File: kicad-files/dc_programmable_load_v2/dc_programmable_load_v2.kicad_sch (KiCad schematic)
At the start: 43 parts, among them J1 DC Jack 12V, J3 Conn_01x04_Socket, Q1 IRF3205, U1 LM358DR, U2 ER_OLEDM0.91_1x-I2C, U3 AP63200WU, U4 DS18B20, U5 S-2050

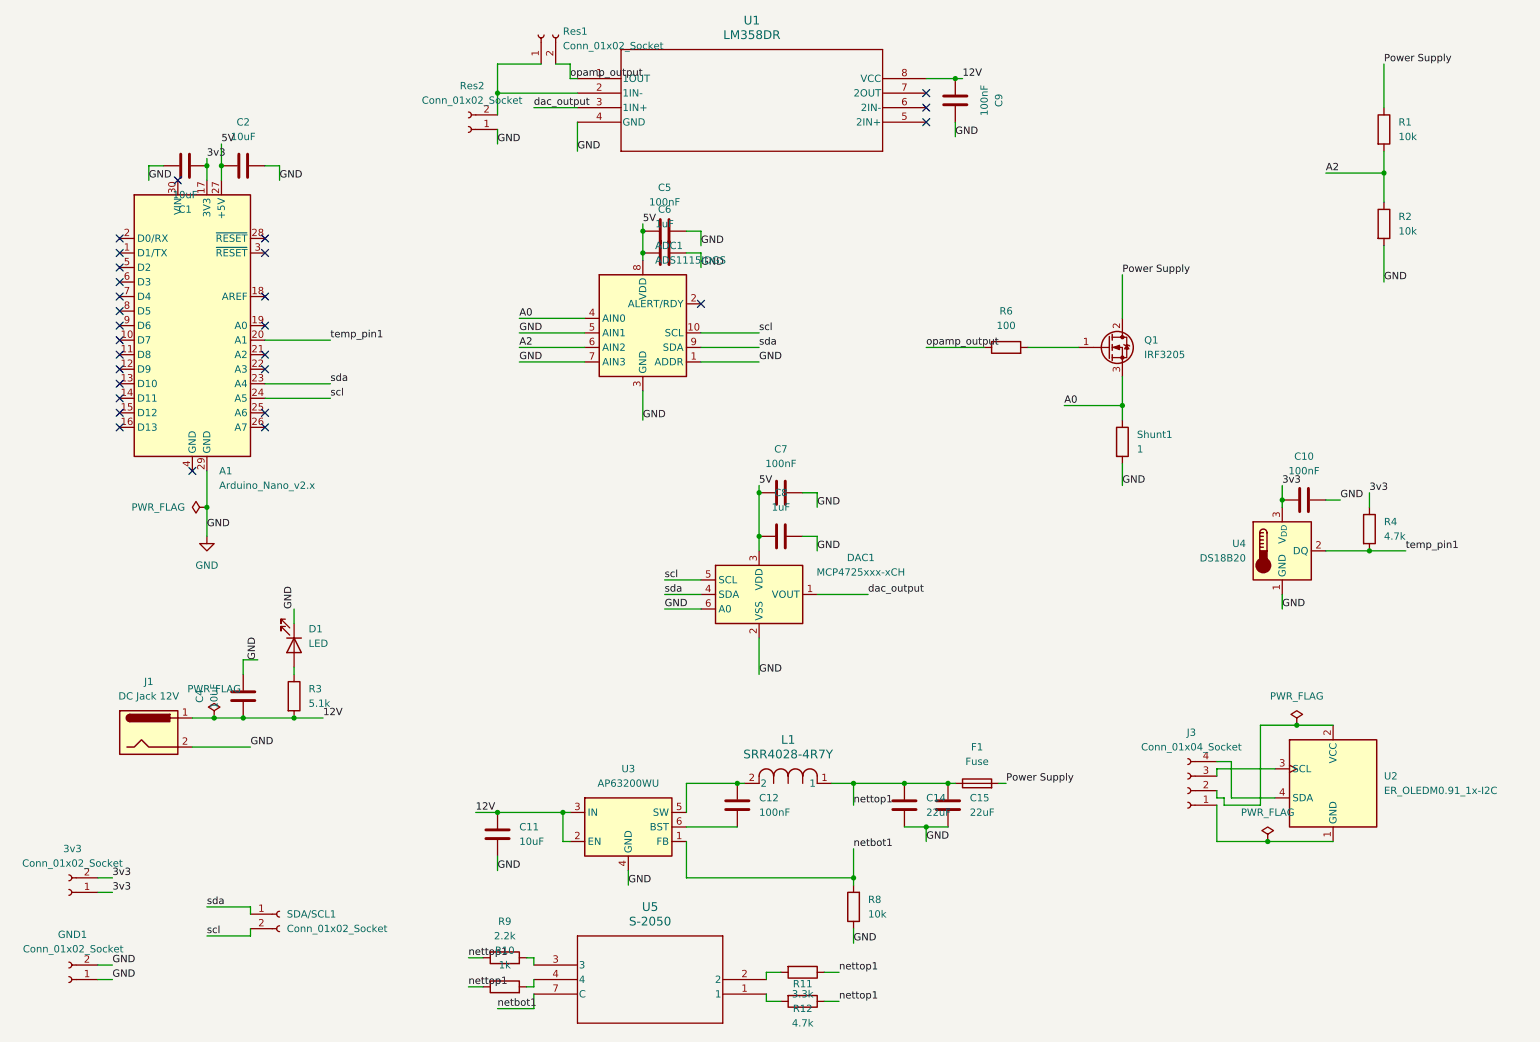
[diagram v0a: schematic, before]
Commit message: anand newest edits
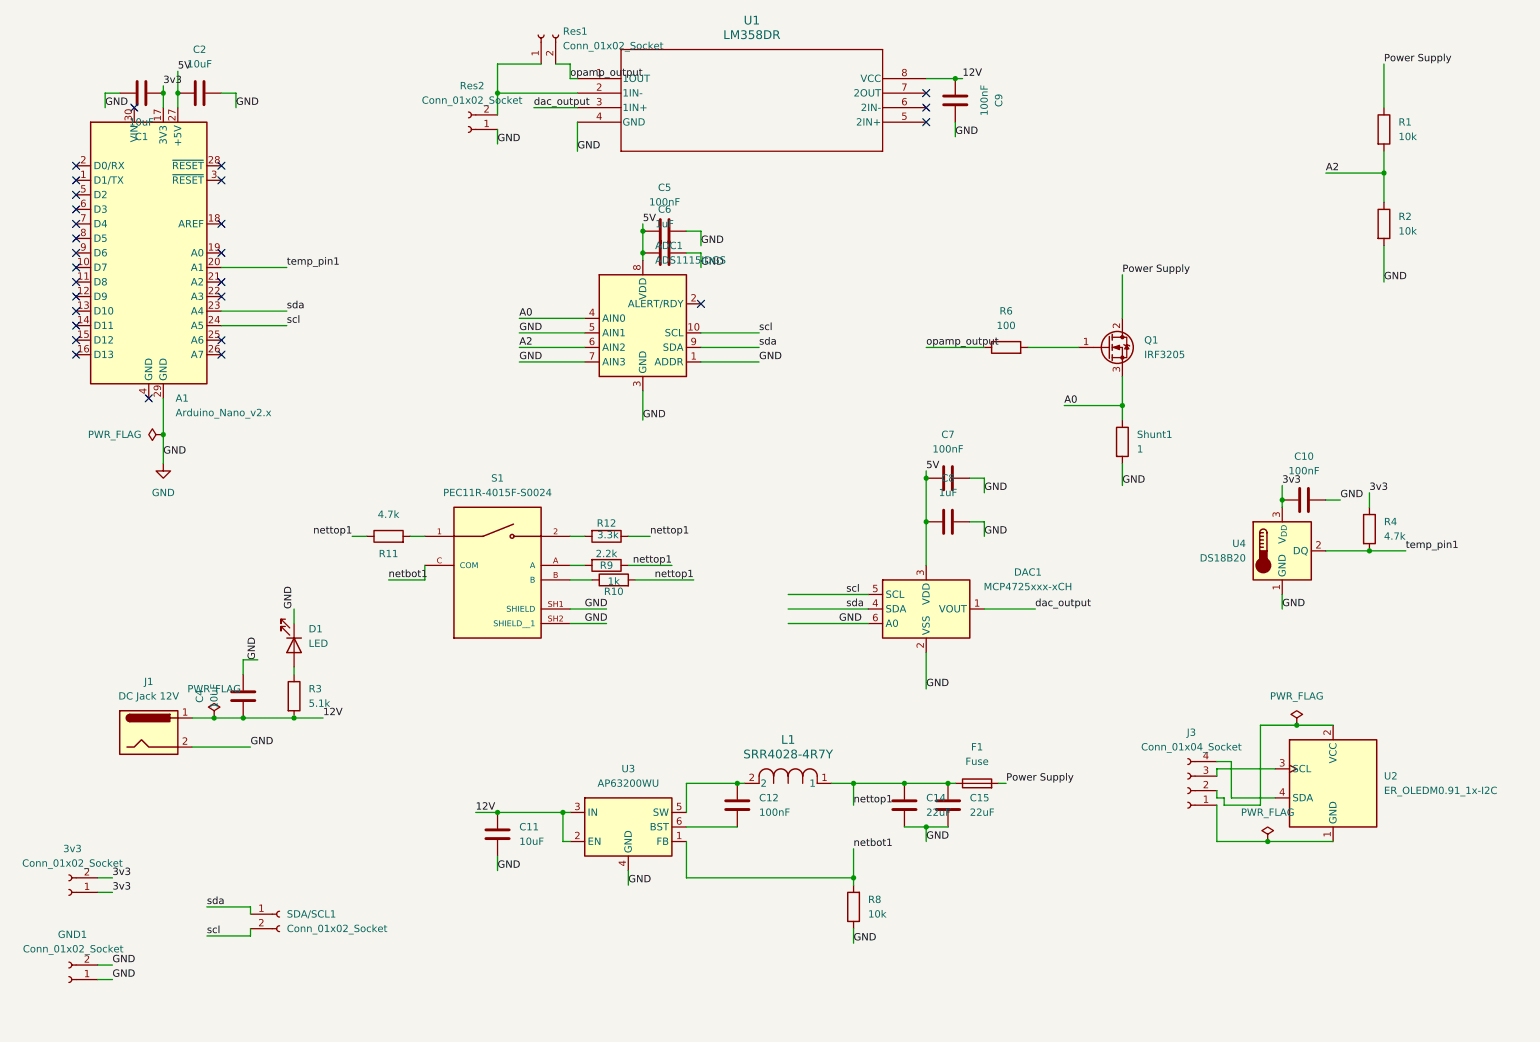
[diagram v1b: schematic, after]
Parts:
- removed U5: S-2050, S-2050_NDC, symbol 2026-07-10_18-54-42:S-2050
- added S1: PEC11R-4015F-S0024, PEC11R-4015F-S0024:XDCR_PEC11R-4015F-S0024, symbol pec:PEC11R-4015F-S0024
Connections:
- net GND: now also S1.SH1 (SHIELD), S1.SH2 (SHIELD__1)
- net netbot1: now also S1.C (COM)
- net nettop1: now also R10.2; no longer R10.1
- net at R11.2: now also S1.1
- net at R12.2: now also S1.2
- net at R9.2: now also S1.A
- new net: R10.1, S1.B
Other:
- moved on the sheet: A1, C1, C2, C7, C8, DAC1, R10, R11, R12, R9
